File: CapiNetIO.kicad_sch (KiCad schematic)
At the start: 92 parts, among them J1 USB_B_Micro, J2 SWD Prg, J3 1963421, J4 USART3, J5 SWD Prg, Q1 MMBT2222A, Q2 MMBT2222A, Q3 MMBT2222A, Q4 MMBT2222A, SW1 SW_SPDT, U1 STM32F446RETx, U3 AMS1117-3.3, Y1 16MHz

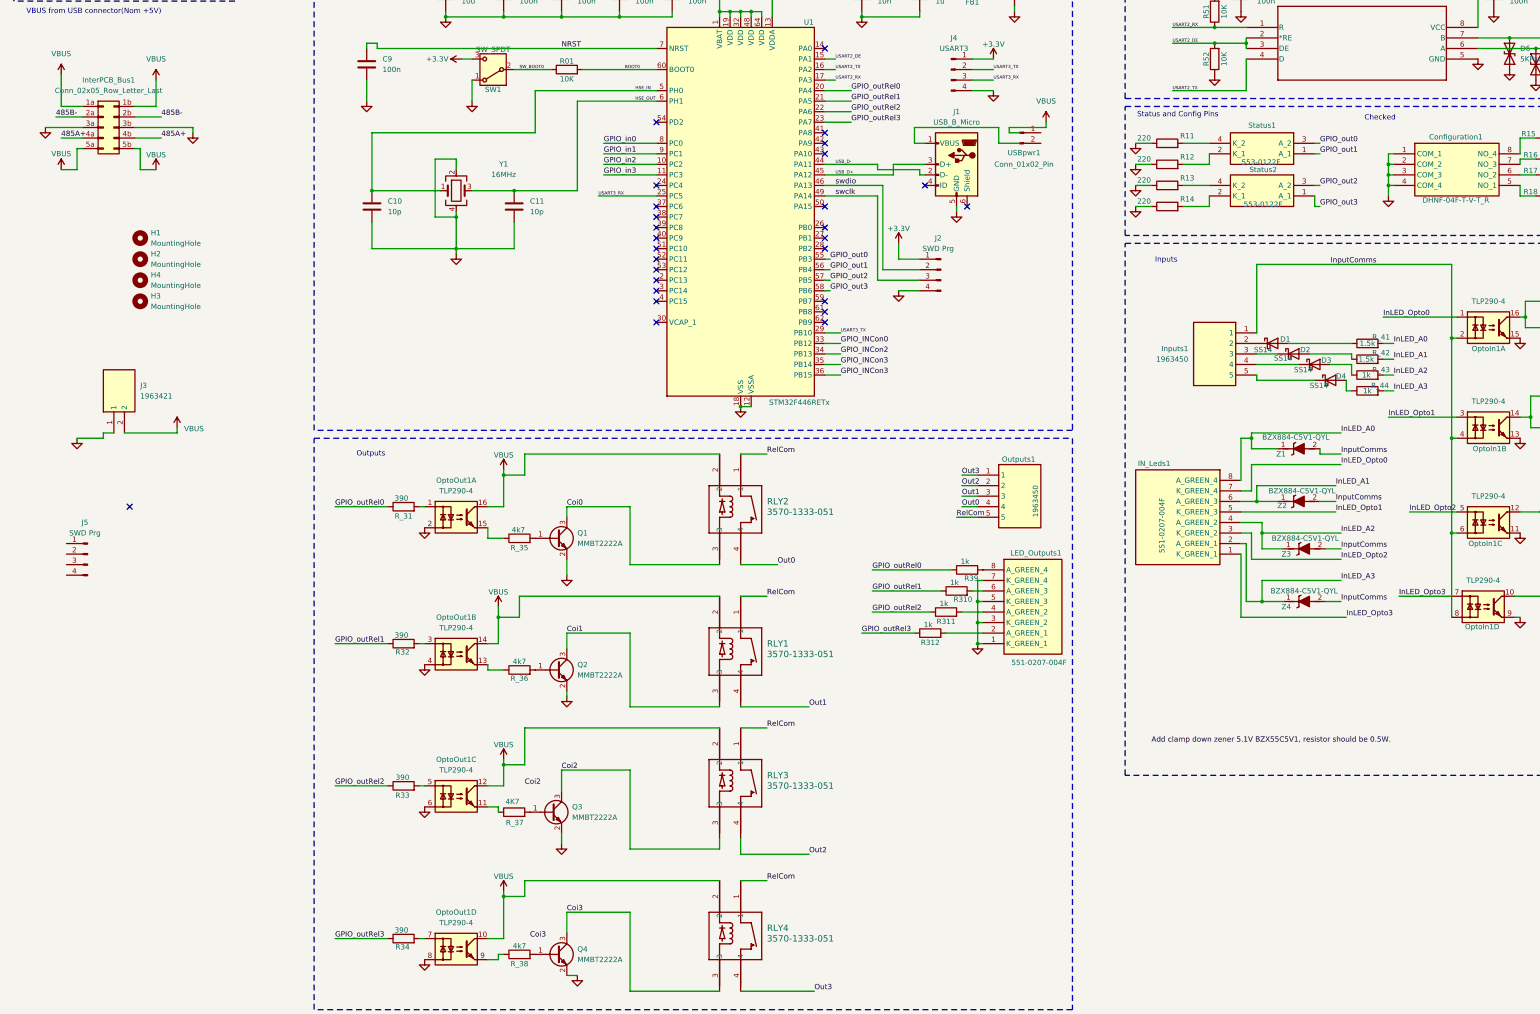
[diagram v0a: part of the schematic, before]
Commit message: Overall Check, need to update the pbc constrains to pass checks
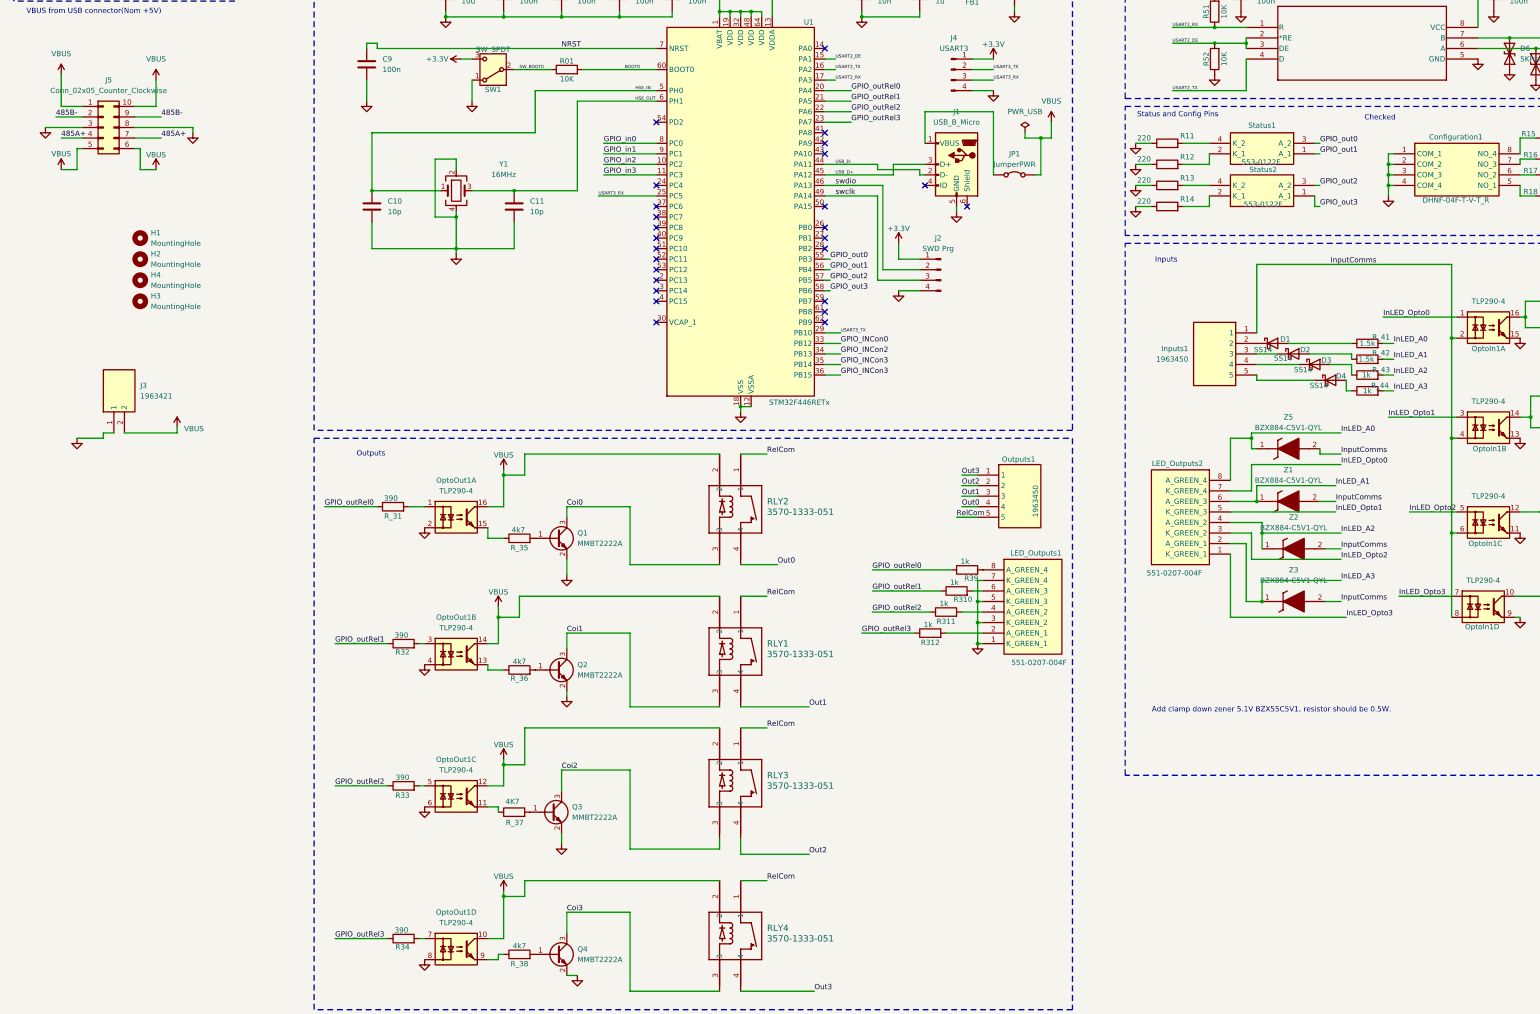
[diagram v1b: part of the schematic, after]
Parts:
- removed IN_Leds1: 551-0207-004F, LED 551 0207 004F:5510207004F, symbol LED Array 551-0207-004F:551-0207-004F
- removed InterPCB_Bus1: Conn_02x05_Row_Letter_Last, Connector_PinHeader_2.54mm:PinHeader_2x05_P2.54mm_Vertical, symbol Connector_Generic:Conn_02x05_Row_Letter_Last
- removed J5: SWD Prg, Connector_PinHeader_1.00mm:PinHeader_1x04_P1.00mm_Vertical, symbol Connector:Conn_01x04_Pin
- removed USBpwr1: Conn_01x02_Pin, Connector_JST:JST_VH_S2P-VH_1x02_P3.96mm_Horizontal, symbol Connector:Conn_01x02_Pin
- removed Z4: BZX884-C5V1-QYL, BZX884C5V1QYL, symbol BZX884-C5V1-QYL_Zener:BZX884-C5V1-QYL
- added J5: Conn_02x05_Counter_Clockwise, Connector_IDC:IDC-Header_2x05_P2.54mm_Vertical, symbol Connector_Generic:Conn_02x05_Counter_Clockwise
- added JP1: JumperPWR, TestPoint:TestPoint_2Pads_Pitch2.54mm_Drill0.8mm, symbol Jumper:Jumper_2_Bridged
- added LED_Outputs2: 551-0207-004F, LED 551 0207 004F:5510207004F, symbol LED Array 551-0207-004F:551-0207-004F
- added Z5: BZX884-C5V1-QYL, BZX884-C5V1-QYL:BZX884C5V1QYL, symbol BZX884-C5V1-QYL_Zener:BZX884-C5V1-QYL
- J2, J4: footprint Connector_PinHeader_1.00mm:PinHeader_1x04_P1.00mm_Vertical -> Connector_PinHeader_2.54mm:PinHeader_1x04_P2.54mm_Horizontal
- J3: footprint 1963421 -> 1963421_2Poles:1963421
- LED_Outputs1: footprint 5510207004F -> LED 551 0207 004F:5510207004F
- RLY1, RLY2, RLY3, RLY4: footprint RELAY4_3570-1333-051_COM -> 3570-1419-054:RELAY4_3570-1333-051_COM
- Z1, Z2, Z3: footprint BZX884C5V1QYL -> BZX884-C5V1-QYL:BZX884C5V1QYL
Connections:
- net 485A+: now also J5.4 (Pin_4), J5.7 (Pin_7)
- net 485B-: now also J5.2 (Pin_2), J5.9 (Pin_9)
- net GND: now also J5.3 (Pin_3), J5.8 (Pin_8)
- net InLED_A0: now also LED_Outputs2.8 (A_GREEN_4), Z5.1 (K); no longer Z1.1 (K)
- net InLED_A1: now also Z1.1 (K), LED_Outputs2.6 (A_GREEN_3); no longer Z2.1 (K)
- net InLED_A2: now also Z2.1 (K), LED_Outputs2.4 (A_GREEN_2); no longer Z3.1 (K)
- net InLED_A3: now also Z3.1 (K), LED_Outputs2.2 (A_GREEN_1)
- net InLED_Opto0: now also LED_Outputs2.7 (K_GREEN_4)
- net InLED_Opto1: now also LED_Outputs2.5 (K_GREEN_3)
- net InLED_Opto2: now also LED_Outputs2.3 (K_GREEN_2)
- net InLED_Opto3: now also LED_Outputs2.1 (K_GREEN_1)
- net InputComms: now also Z5.2 (A)
- net VBUS: now also J5.1 (Pin_1), J5.10 (Pin_10), J5.5 (Pin_5), J5.6 (Pin_6), JP1.2 (B)
- net at J1.1 (VBUS): now also JP1.1 (A)
- no-connect marks 27 -> 26
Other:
- note added: "Add clamp down zener 5.1V BZX55C5V1, resistor should be 0.5W."
- moved on the sheet: R_31

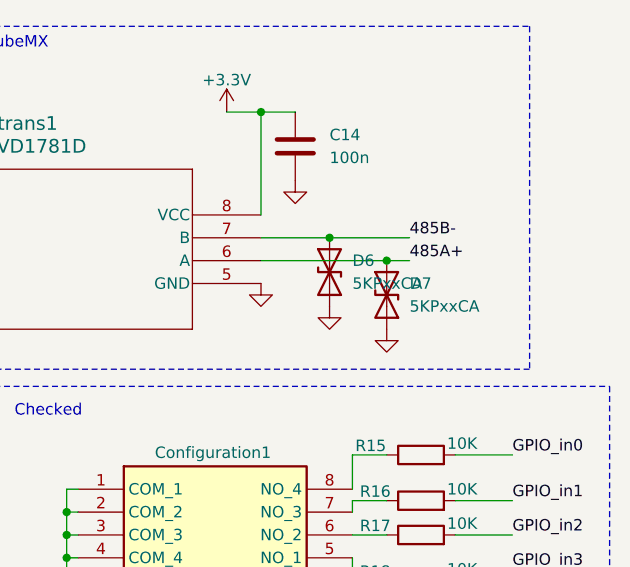
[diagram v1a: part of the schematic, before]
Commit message: Checked footprints and pcb constrains, time to start tracing
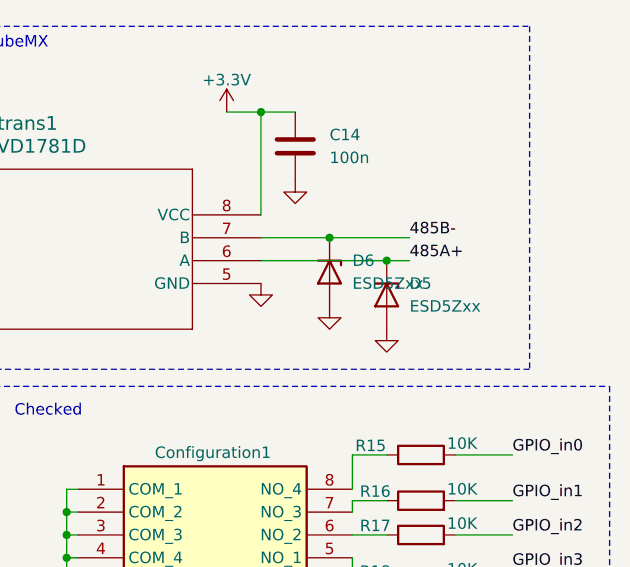
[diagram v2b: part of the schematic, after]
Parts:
- removed D6, D7: 5KPxxCA, Diode_THT:D_P600_R-6_P20.00mm_Horizontal, symbol Diode:5KPxxCA
- added D5, D6: ESD5Zxx, Diode_SMD:D_SOD-523, symbol Diode:ESD5Zxx
- C1, C10, C11, C14, C15, C2, C3, C4: footprint Capacitor_SMD:C_01005_0402Metric -> Capacitor_SMD:C_0603_1608Metric
- C6, C7, C8, C9: footprint Capacitor_SMD:C_0402_1005Metric -> Capacitor_SMD:C_0603_1608Metric
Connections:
- net 485A+: now also D5.1 (K)
- net 485B-: now also D6.1 (K)
- net GND: now also D5.2 (A), D6.2 (A)
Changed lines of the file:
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@@
 	)
 	(junction
-		(at 374.65 49.53)
-		(diameter 0)
-		(color 0 0 0 0)
-	)
-	(junction
 		(at 160.02 44.45)
 		(diameter 0)
@@
 	)
 	(junction
+		(at 374.65 49.53)
+		(diameter 0)
+		(color 0 0 0 0)
+	)
+	(junction
 		(at 360.68 168.91)
 		(diameter 0)
@@
 	)
 	(junction
+		(at 381 52.07)
+		(diameter 0)
+		(color 0 0 0 0)
+	)
+	(junction
 		(at 189.23 43.18)
 		(diameter 0)
@@
 		(color 0 0 0 0)
 	)
-	(junction
-		(at 381 52.07)
-		(diameter 0)
-		(color 0 0 0 0)
-	)
 	(no_connect
 		(at 209.55 115.57)
@@
 	(wire
 		(pts
+			(xy 374.65 49.53) (xy 383.54 49.53)
+		)
+		(stroke
+			(width 0)
+			(type default)
+		)
+	)
+	(wire
+		(pts
 			(xy 186.69 44.45) (xy 186.69 43.18)
 		)
@@
 	(wire
 		(pts
+			(xy 381 52.07) (xy 383.54 52.07)
+		)
+		(stroke
+			(width 0)
+			(type default)
+		)
+	)
+	(wire
+		(pts
 			(xy 162.56 193.04) (xy 147.32 193.04)
 		)
@@
 	(wire
 		(pts
-			(xy 381 52.07) (xy 383.54 52.07)
-		)
-		(stroke
-			(width 0)
-			(type default)
-		)
-	)
-	(wire
-		(pts
 			(xy 154.94 87.63) (xy 168.91 87.63)
 		)
@@
 	(wire
 		(pts
-			(xy 374.65 49.53) (xy 383.54 49.53)
-		)
-		(stroke
-			(width 0)
-			(type default)
-		)
-	)
-	(wire
-		(pts
 			(xy 284.48 90.17) (xy 288.29 90.17)
 		)
@@
 			)
 		)
-		(property "Footprint" "Capacitor_SMD:C_0402_1005Metric"
+		(property "Footprint" "Capacitor_SMD:C_0603_1608Metric"
 			(at 219.4052 43.18 0)
 			(effects
@@
 	)
 	(symbol
-		(lib_id "Diode:5KPxxCA")
-		(at 374.65 53.34 90)
-		(unit 1)
-		(exclude_from_sim no)
-		(in_bom yes)
-		(on_board yes)
-		(dnp no)
-		(fields_autoplaced yes)
-		(property "Reference" "D6"
-			(at 377.19 52.0699 90)
-			(effects
-				(font
-					(size 1.27 1.27)
-				)
-				(justify right)
-			)
-		)
-		(property "Value" "5KPxxCA"
-			(at 377.19 54.6099 90)
-			(effects
-				(font
-					(size 1.27 1.27)
-				)
-				(justify right)
-			)
-		)
-		(property "Footprint" "Diode_THT:D_P600_R-6_P20.00mm_Horizontal"
-			(at 379.73 53.34 0)
-			(effects
-				(font
-					(size 1.27 1.27)
-				)
-				(hide yes)
-			)
-		)
-		(property "Datasheet" "https://diotec.com/tl_files/diotec/files/pdf/datasheets/5kp65.pdf"
-			(at 374.65 53.34 0)
-			(effects
-				(font
-					(size 1.27 1.27)
-				)
-				(hide yes)
-			)
-		)
-		(property "Description" "5000W bidirectional Transient Voltage Suppressor, P-600"
-			(at 374.65 53.34 0)
-			(effects
-				(font
-					(size 1.27 1.27)
-				)
-				(hide yes)
-			)
-		)
-		(pin "2"
-		)
-		(pin "1"
-		)
-		(instances
-			(project ""
-				(path "/1a5652bf-ba49-4248-8cd9-02a29183ef4e"
-					(reference "D6")
-					(unit 1)
-				)
-			)
-		)
-	)
-	(symbol
 		(lib_id "Device:R")
 		(at 234.95 193.04 90)
@@
 			)
 		)
-		(property "Footprint" "Capacitor_SMD:C_01005_0402Metric"
+		(property "Footprint" "Capacitor_SMD:C_0603_1608Metric"
 			(at 147.0152 43.18 0)
 			(effects
@@
 			)
 		)
-		(property "Footprint" "Capacitor_SMD:C_0402_1005Metric"
+		(property "Footprint" "Capacitor_SMD:C_0603_1608Metric"
 			(at 100.0252 59.69 0)
 			(effects
@@
 			)
 		)
-		(property "Footprint" "Capacitor_SMD:C_0402_1005Metric"
+		(property "Footprint" "Capacitor_SMD:C_0603_1608Metric"
 			(at 233.3752 43.18 0)
 			(effects
@@
 			)
 		)
-		(property "Footprint" "Capacitor_SMD:C_01005_0402Metric"
+		(property "Footprint" "Capacitor_SMD:C_0603_1608Metric"
 			(at 101.2952 93.98 0)
 			(effects
@@
 			)
 		)
-		(property "Footprint" "Capacitor_SMD:C_01005_0402Metric"
+		(property "Footprint" "Capacitor_SMD:C_0603_1608Metric"
 			(at 160.9852 43.18 0)
 			(effects
@@
 			)
 		)
-		(property "Footprint" "Capacitor_SMD:C_01005_0402Metric"
+		(property "Footprint" "Capacitor_SMD:C_0603_1608Metric"
 			(at 371.8052 43.18 0)
 			(effects
@@
 			)
 		)
-		(property "Footprint" "Capacitor_SMD:C_01005_0402Metric"
+		(property "Footprint" "Capacitor_SMD:C_0603_1608Metric"
 			(at 135.5852 93.98 0)
 			(effects
@@
 	)
 	(symbol
+		(lib_id "Diode:ESD5Zxx")
+		(at 381 55.88 270)
+		(unit 1)
+		(exclude_from_sim no)
+		(in_bom yes)
+		(on_board yes)
+		(dnp no)
+		(fields_autoplaced yes)
+		(property "Reference" "D5"
+			(at 383.54 54.6099 90)
+			(effects
+				(font
+					(size 1.27 1.27)
+				)
+				(justify left)
+			)
+		)
+		(property "Value" "ESD5Zxx"
+			(at 383.54 57.1499 90)
+			(effects
+				(font
+					(size 1.27 1.27)
+				)
+				(justify left)
+			)
+		)
+		(property "Footprint" "Diode_SMD:D_SOD-523"
+			(at 376.555 55.88 0)
+			(effects
+				(font
+					(size 1.27 1.27)
+				)
+				(hide yes)
+			)
+		)
+		(property "Datasheet" "https://www.onsemi.com/pdf/datasheet/esd5z2.5t1-d.pdf"
+			(at 381 55.88 0)
+			(effects
+				(font
+					(size 1.27 1.27)
+				)
+				(hide yes)
+			)
+		)
+		(property "Description" "ESD Protection Diode, SOD-523"
+			(at 381 55.88 0)
+			(effects
+				(font
+					(size 1.27 1.27)
+				)
+				(hide yes)
+			)
+		)
+		(pin "2"
+		)
+		(pin "1"
+		)
+		(instances
+			(project ""
+				(path "/1a5652bf-ba49-4248-8cd9-02a29183ef4e"
+					(reference "D5")
+					(unit 1)
+				)
+			)
+		)
+	)
+	(symbol
 		(lib_id "power:GND")
 		(at 218.44 44.45 0)
@@
 	)
 	(symbol
+		(lib_id "Diode:ESD5Zxx")
+		(at 374.65 53.34 270)
+		(unit 1)
+		(exclude_from_sim no)
+		(in_bom yes)
+		(on_board yes)
+		(dnp no)
+		(fields_autoplaced yes)
+		(property "Reference" "D6"
+			(at 377.19 52.0699 90)
+			(effects
+				(font
+					(size 1.27 1.27)
+				)
+				(justify left)
+			)
+		)
+		(property "Value" "ESD5Zxx"
+			(at 377.19 54.6099 90)
+			(effects
+				(font
+					(size 1.27 1.27)
+				)
+				(justify left)
+			)
+		)
+		(property "Footprint" "Diode_SMD:D_SOD-523"
+			(at 370.205 53.34 0)
+			(effects
+				(font
+					(size 1.27 1.27)
+				)
+				(hide yes)
+			)
+		)
+		(property "Datasheet" "https://www.onsemi.com/pdf/datasheet/esd5z2.5t1-d.pdf"
+			(at 374.65 53.34 0)
+			(effects
+				(font
+					(size 1.27 1.27)
+				)
+				(hide yes)
+			)
+		)
+		(property "Description" "ESD Protection Diode, SOD-523"
+			(at 374.65 53.34 0)
+			(effects
+				(font
+					(size 1.27 1.27)
+				)
+				(hide yes)
+			)
+		)
+		(pin "2"
+		)
+		(pin "1"
+		)
+		(instances
+			(project "CapiNetIO"
+				(path "/1a5652bf-ba49-4248-8cd9-02a29183ef4e"
+					(reference "D6")
+					(unit 1)
+				)
+			)
+		)
+	)
+	(symbol
 		(lib_id "power:+3.3V")
 		(at 363.22 35.56 0)
@@
 			)
 		)
-		(property "Footprint" "Capacitor_SMD:C_0402_1005Metric"
+		(property "Footprint" "Capacitor_SMD:C_0603_1608Metric"
 			(at 256.2352 41.91 0)
 			(effects
@@
 			)
 		)
-		(property "Footprint" "Capacitor_SMD:C_01005_0402Metric"
+		(property "Footprint" "Capacitor_SMD:C_0603_1608Metric"
 			(at 173.6852 43.18 0)
 			(effects
@@
 	)
 	(symbol
-		(lib_id "Diode:5KPxxCA")
-		(at 381 55.88 90)
-		(unit 1)
-		(exclude_from_sim no)
-		(in_bom yes)
-		(on_board yes)
-		(dnp no)
-		(fields_autoplaced yes)
-		(property "Reference" "D7"
-			(at 383.54 54.6099 90)
-			(effects
-				(font
-					(size 1.27 1.27)
-				)
-				(justify right)
-			)
-		)
-		(property "Value" "5KPxxCA"
-			(at 383.54 57.1499 90)
-			(effects
-				(font
-					(size 1.27 1.27)
-				)
-				(justify right)
-			)
-		)
-		(property "Footprint" "Diode_THT:D_P600_R-6_P20.00mm_Horizontal"
-			(at 386.08 55.88 0)
-			(effects
-				(font
-					(size 1.27 1.27)
-				)
-				(hide yes)
-			)
-		)
-		(property "Datasheet" "https://diotec.com/tl_files/diotec/files/pdf/datasheets/5kp65.pdf"
-			(at 381 55.88 0)
-			(effects
-				(font
-					(size 1.27 1.27)
-				)
-				(hide yes)
-			)
-		)
-		(property "Description" "5000W bidirectional Transient Voltage Suppressor, P-600"
-			(at 381 55.88 0)
-			(effects
-				(font
-					(size 1.27 1.27)
-				)
-				(hide yes)
-			)
-		)
-		(pin "2"
-		)
-		(pin "1"
-		)
-		(instances
-			(project "CapiNetIO"
-				(path "/1a5652bf-ba49-4248-8cd9-02a29183ef4e"
-					(reference "D7")
-					(unit 1)
-				)
-			)
-		)
-	)
-	(symbol
 		(lib_id "Device:R")
 		(at 384.81 73.66 90)
@@
 			)
 		)
-		(property "Footprint" "Capacitor_SMD:C_01005_0402Metric"
+		(property "Footprint" "Capacitor_SMD:C_0603_1608Metric"
 			(at 133.0452 43.18 0)
 			(effects
@@
 			)
 		)
-		(property "Footprint" "Capacitor_SMD:C_01005_0402Metric"
+		(property "Footprint" "Capacitor_SMD:C_0603_1608Metric"
 			(at 310.8452 43.18 0)
 			(effects
